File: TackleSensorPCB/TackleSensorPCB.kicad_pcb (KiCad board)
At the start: 2 copper layers, 60 x 25 mm, 24 parts, among them J1 PJ-037A, J2 Conn_01x03_Male, J3 Conn_01x04_Male, J4 Conn_01x07_Male, Q1 2N7002, Q2 2N7002, SW1 SW_DPST_x2, U1 TPS62172DSG, U2 MSP430FR2433IRGER, U3 LIS2DH12TR

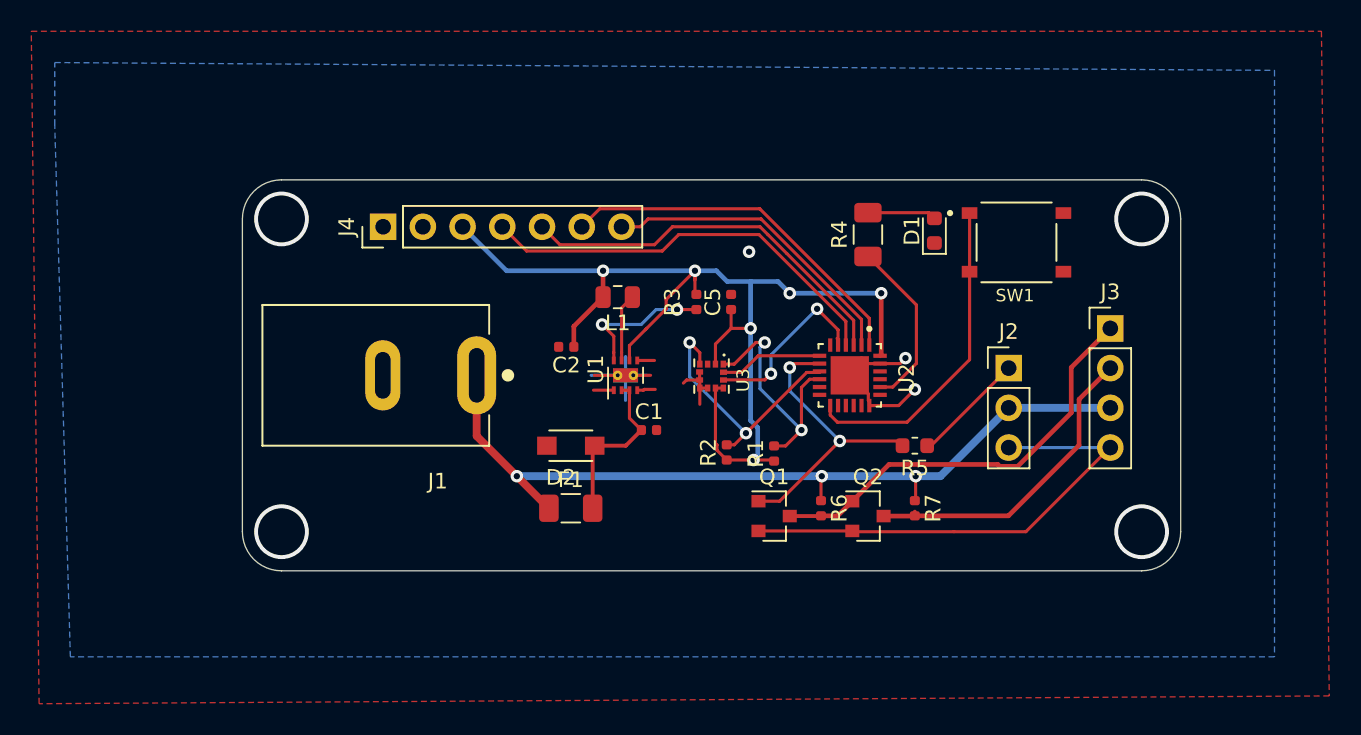
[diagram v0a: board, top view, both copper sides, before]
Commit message: Completed 3D model
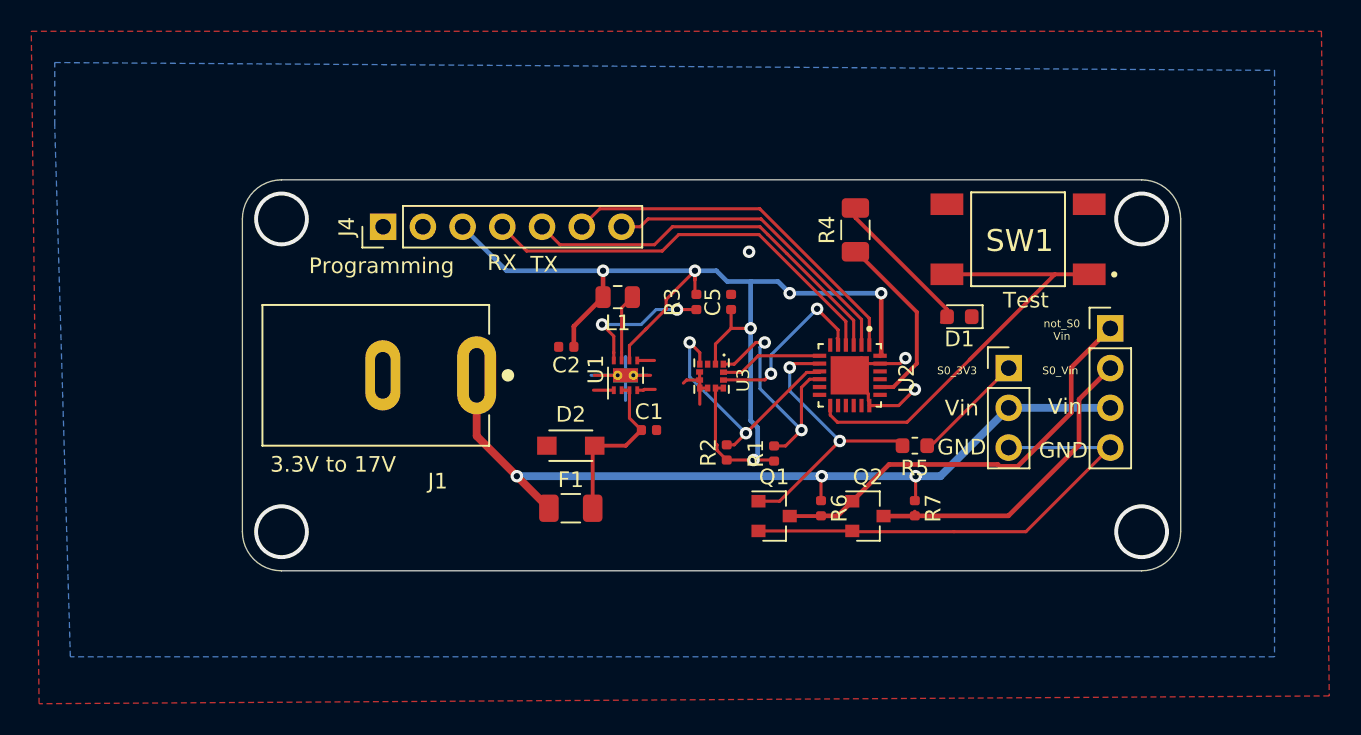
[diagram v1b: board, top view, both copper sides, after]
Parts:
- SW1: value SW_DPST_x2 -> FSM4JSMA; footprint TS-1187A-B-A-B:SW_TS-1187A-B-A-B -> FSM4JSMA:TE_FSM4JSMA
- moved D1 5.73 mm to (124.8, 67.8), turned to 180 degrees
- moved R4 0.85 mm to (118.2, 62.2)
- moved SW1 0.22 mm to (128.6, 62.8), turned to 180 degrees
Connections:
- SW1 pad 2: GND -> SW0
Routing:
- net SW0: track 20.7 -> 28.2 mm
- net Net-(D1-Pad2): track 4.40 -> 9.89 mm
- net L0: track 11.1 -> 11.8 mm
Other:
- board text added: "3.3V to 17V"
- board text added: "GND"
- board text added: "Programming"
- board text added: "RX"
- board text added: "S0_3V3"
- board text added: "S0_Vin"
- board text added: "TX"
- board text added: "Test"
- board text added: "Vin"
- board text added: "not_S0 Vin"
